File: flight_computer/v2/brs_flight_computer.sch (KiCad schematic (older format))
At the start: 0 parts

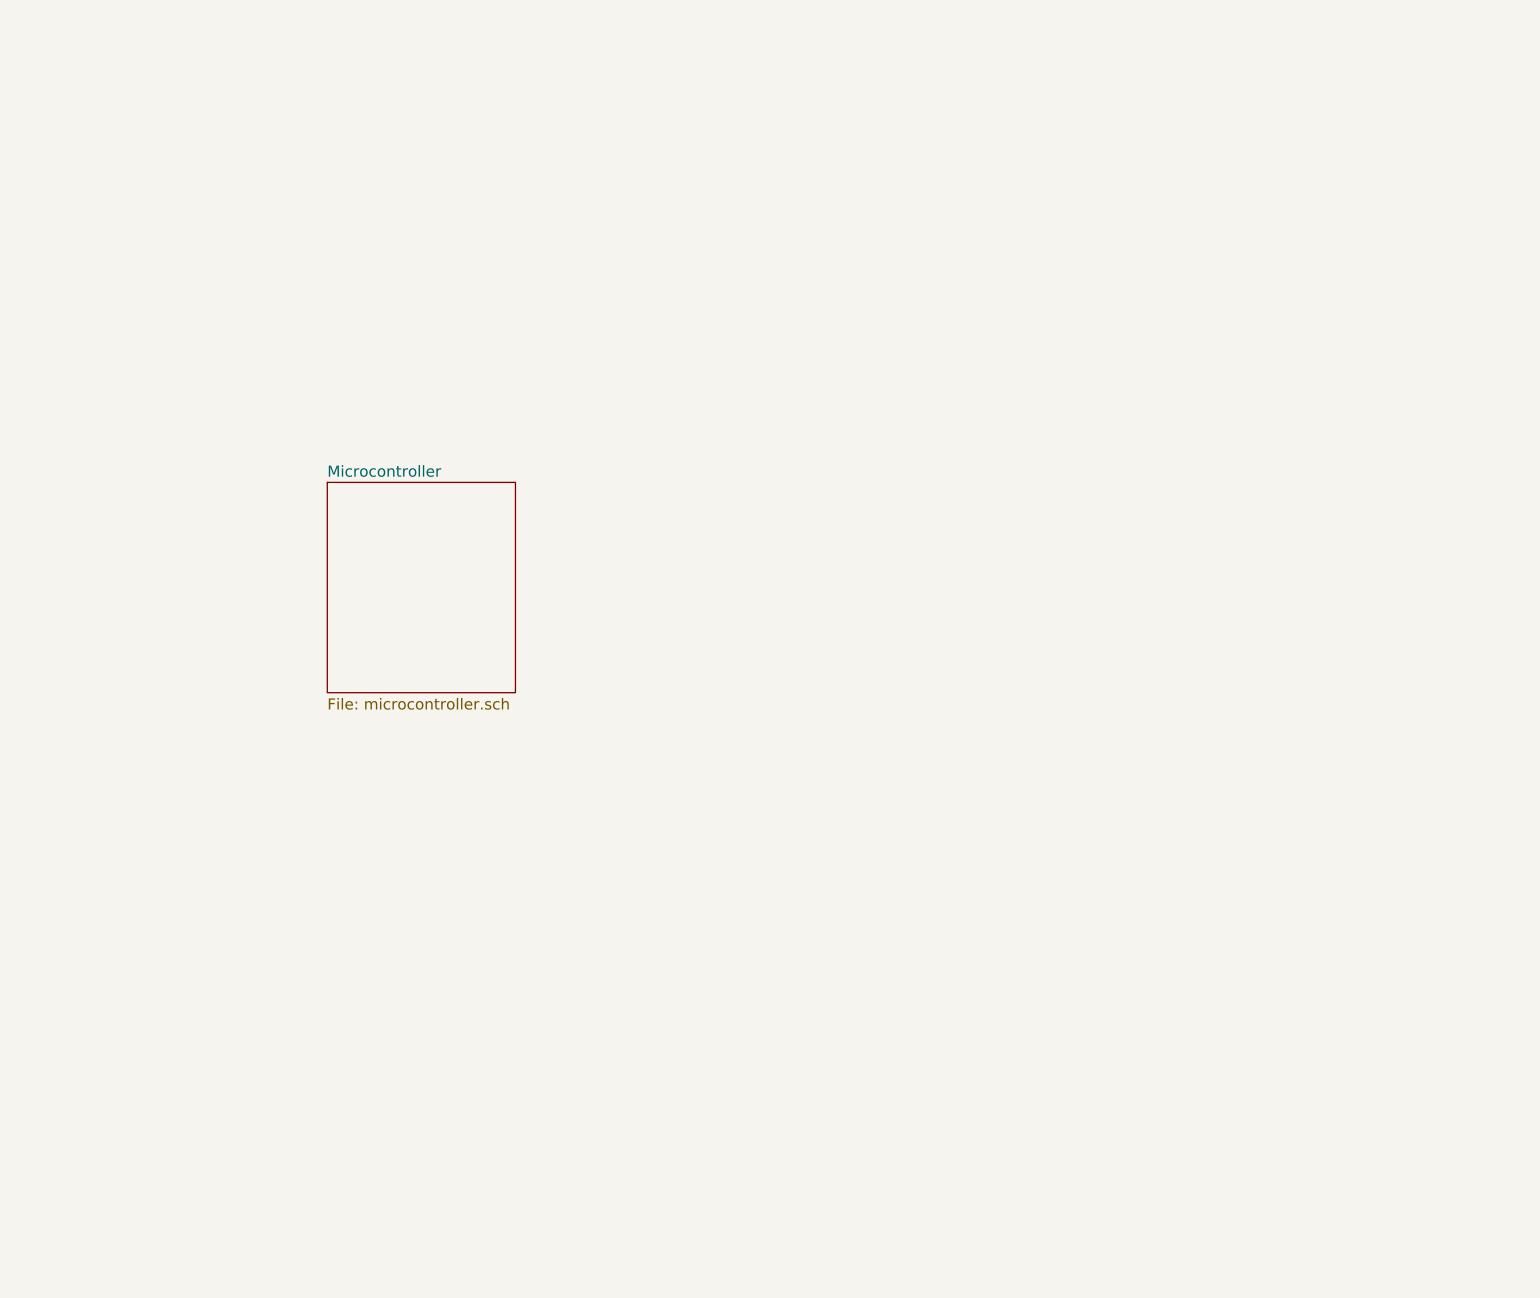
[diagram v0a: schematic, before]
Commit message: Nearing first pass layout for Rev B flight computer
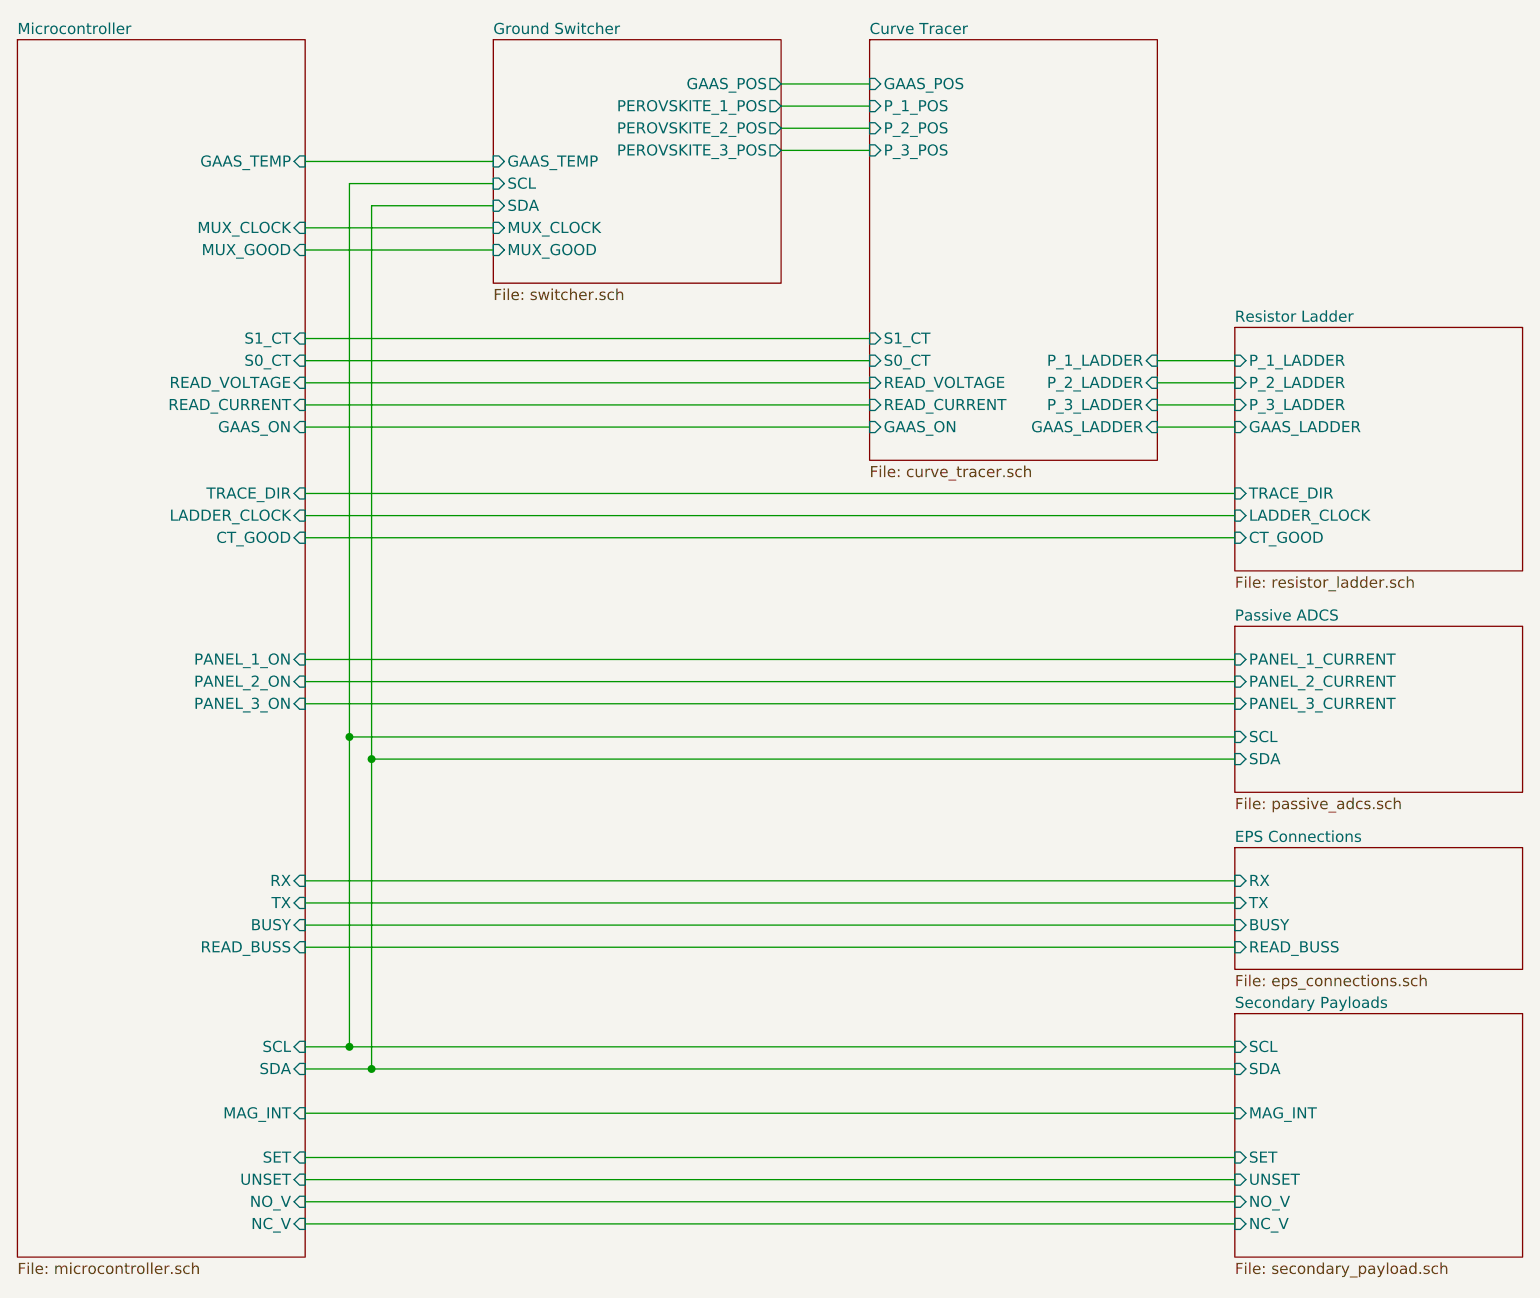
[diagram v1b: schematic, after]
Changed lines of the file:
@@
 $Descr A4 11693 8268
 encoding utf-8
-Sheet 1 2
-Title ""
-Date ""
-Rev ""
-Comp ""
-Comment1 ""
-Comment2 ""
-Comment3 ""
-Comment4 ""
+Sheet 1 8
+Title "Big Red Satellite Flight Computer - Top Level"
+Date "2023-08-13"
+Rev "B"
+Comp "UNL Aerospace Club | Advanced eXperimental Payloads"
+Comment1 "Copyright (c) 2023"
+Comment2 "Designer: WSA"
+Comment3 "Reviewer:"
+Comment4 "Approved:"
 $EndDescr
 $Sheet
-S 3850 2800 850  950
+S 2450 800  1300 5500
 U 64AE160A
 F0 "Microcontroller" 50
 F1 "microcontroller.sch" 50
-$EndSheet
+F2 "READ_CURRENT" I R 3750 2450 50
+F3 "READ_VOLTAGE" I R 3750 2350 50
+F4 "S0_CT" I R 3750 2250 50
+F5 "S1_CT" I R 3750 2150 50
+F6 "GAAS_ON" I R 3750 2550 50
+F7 "MUX_CLOCK" I R 3750 1650 50
+F8 "MUX_GOOD" I R 3750 1750 50
+F9 "GAAS_TEMP" I R 3750 1350 50
+F10 "LADDER_CLOCK" I R 3750 2950 50
+F11 "TRACE_DIR" I R 3750 2850 50
+F12 "CT_GOOD" I R 3750 3050 50
+F13 "PANEL_1_ON" I R 3750 3600 50
+F14 "PANEL_2_ON" I R 3750 3700 50
+F15 "PANEL_3_ON" I R 3750 3800 50
+F16 "SCL" I R 3750 5350 50
+F17 "SDA" I R 3750 5450 50
+F18 "BUSY" I R 3750 4800 50
+F19 "RX" I R 3750 4600 50
+F20 "TX" I R 3750 4700 50
+F21 "MAG_INT" I R 3750 5650 50
+F22 "SET" I R 3750 5850 50
+F23 "UNSET" I R 3750 5950 50
+F24 "NO_V" I R 3750 6050 50
+F25 "NC_V" I R 3750 6150 50
+F26 "READ_BUSS" I R 3750 4900 50
+$EndSheet
+$Sheet
+S 6300 800  1300 1900
+U 64D8220D
+F0 "Curve Tracer" 50
+F1 "curve_tracer.sch" 50
+F2 "GAAS_POS" I L 6300 1000 50
+F3 "GAAS_LADDER" I R 7600 2550 50
+F4 "GAAS_ON" I L 6300 2550 50
+F5 "P_1_POS" I L 6300 1100 50
+F6 "P_1_LADDER" I R 7600 2250 50
+F7 "P_2_POS" I L 6300 1200 50
+F8 "P_2_LADDER" I R 7600 2350 50
+F9 "P_3_POS" I L 6300 1300 50
+F10 "P_3_LADDER" I R 7600 2450 50
+F11 "READ_CURRENT" I L 6300 2450 50
+F12 "READ_VOLTAGE" I L 6300 2350 50
+F13 "S0_CT" I L 6300 2250 50
+F14 "S1_CT" I L 6300 2150 50
+$EndSheet
+$Sheet
+S 7950 3450 1300 750
+U 64D823E8
+F0 "Passive ADCS" 50
+F1 "passive_adcs.sch" 50
+F2 "PANEL_1_CURRENT" I L 7950 3600 50
+F3 "PANEL_2_CURRENT" I L 7950 3700 50
+F4 "PANEL_3_CURRENT" I L 7950 3800 50
+F5 "SCL" I L 7950 3950 50
+F6 "SDA" I L 7950 4050 50
+$EndSheet
+$Sheet
+S 7950 2100 1300 1100
+U 64D82674
+F0 "Resistor Ladder" 50
+F1 "resistor_ladder.sch" 50
+F2 "P_2_LADDER" I L 7950 2350 50
+F3 "P_3_LADDER" I L 7950 2450 50
+F4 "P_1_LADDER" I L 7950 2250 50
+F5 "GAAS_LADDER" I L 7950 2550 50
+F6 "LADDER_CLOCK" I L 7950 2950 50
+F7 "TRACE_DIR" I L 7950 2850 50
+F8 "CT_GOOD" I L 7950 3050 50
+$EndSheet
+$Sheet
+S 4600 800  1300 1100
+U 64D827F9
+F0 "Ground Switcher" 50
+F1 "switcher.sch" 50
+F2 "MUX_CLOCK" I L 4600 1650 50
+F3 "MUX_GOOD" I L 4600 1750 50
+F4 "PEROVSKITE_1_POS" O R 5900 1100 50
+F5 "PEROVSKITE_2_POS" O R 5900 1200 50
+F6 "PEROVSKITE_3_POS" O R 5900 1300 50
+F7 "GAAS_POS" O R 5900 1000 50
+F8 "SDA" I L 4600 1550 50
+F9 "SCL" I L 4600 1450 50
+F10 "GAAS_TEMP" I L 4600 1350 50
+$EndSheet
+Wire Wire Line
+	7950 2250 7600 2250
+Wire Wire Line
+	7600 2350 7950 2350
+Wire Wire Line
+	7950 2450 7600 2450
+Wire Wire Line
+	7600 2550 7950 2550
+Wire Wire Line
+	5900 1000 6300 1000
+Wire Wire Line
+	6300 1100 5900 1100
+Wire Wire Line
+	5900 1200 6300 1200
+Wire Wire Line
+	6300 1300 5900 1300
+$Sheet
+S 7950 4450 1300 550
+U 64D821F3
+F0 "EPS Connections" 50
+F1 "eps_connections.sch" 50
+F2 "RX" I L 7950 4600 50
+F3 "TX" I L 7950 4700 50
+F4 "BUSY" I L 7950 4800 50
+F5 "READ_BUSS" I L 7950 4900 50
+$EndSheet
+$Sheet
+S 7950 5200 1300 1100
+U 6685FD81
+F0 "Secondary Payloads" 50
+F1 "secondary_payload.sch" 50
+F2 "SCL" I L 7950 5350 50
+F3 "SDA" I L 7950 5450 50
+F4 "MAG_INT" I L 7950 5650 50
+F5 "SET" I L 7950 5850 50
+F6 "UNSET" I L 7950 5950 50
+F7 "NO_V" I L 7950 6050 50
+F8 "NC_V" I L 7950 6150 50
+$EndSheet
+Wire Wire Line
+	4600 1350 3750 1350
+Wire Wire Line
+	3750 1650 4600 1650
+Wire Wire Line
+	4600 1750 3750 1750
+Wire Wire Line
+	3750 2150 6300 2150
+Wire Wire Line
+	6300 2250 3750 2250
+Wire Wire Line
+	3750 2350 6300 2350
+Wire Wire Line
+	6300 2450 3750 2450
+Wire Wire Line
+	3750 2550 6300 2550
+Wire Wire Line
+	3750 2850 7950 2850
+Wire Wire Line
+	3750 2950 7950 2950
+Wire Wire Line
+	7950 3050 3750 3050
+Wire Wire Line
+	3750 3600 7950 3600
+Wire Wire Line
+	7950 3700 3750 3700
+Wire Wire Line
+	3750 3800 7950 3800
+Wire Wire Line
+	3750 4600 7950 4600
+Wire Wire Line
+	3750 4700 7950 4700
+Wire Wire Line
+	7950 4800 3750 4800
+Wire Wire Line
+	3750 5350 3950 5350
+Wire Wire Line
+	7950 5450 4050 5450
+Wire Wire Line
+	3750 5650 7950 5650
+Wire Wire Line
+	4600 1450 3950 1450
+Connection ~ 3950 5350
+Wire Wire Line
+	3950 5350 7950 5350
+Wire Wire Line
+	4600 1550 4050 1550
+Wire Wire Line
+	4050 1550 4050 4050
+Connection ~ 4050 5450
+Wire Wire Line
+	4050 5450 3750 5450
+Wire Wire Line
+	7950 3950 3950 3950
+Wire Wire Line
+	3950 1450 3950 3950
+Connection ~ 3950 3950
+Wire Wire Line
+	3950 3950 3950 5350
+Wire Wire Line
+	7950 4050 4050 4050
+Connection ~ 4050 4050
+Wire Wire Line
+	4050 4050 4050 5450
+Wire Wire Line
+	7950 5850 3750 5850
+Wire Wire Line
+	3750 5950 7950 5950
+Wire Wire Line
+	7950 6050 3750 6050
+Wire Wire Line
+	3750 6150 7950 6150
+Wire Wire Line
+	3750 4900 7950 4900
 $EndSCHEMATC

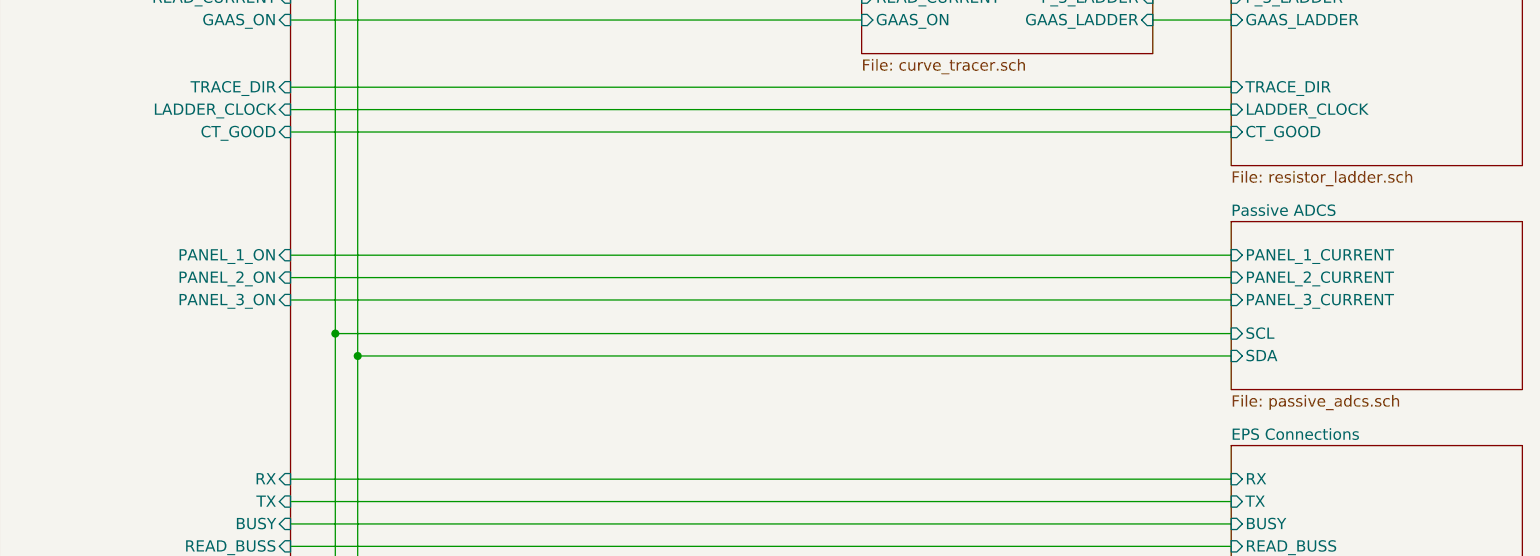
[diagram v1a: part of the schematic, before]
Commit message: Finished layout of flight computer
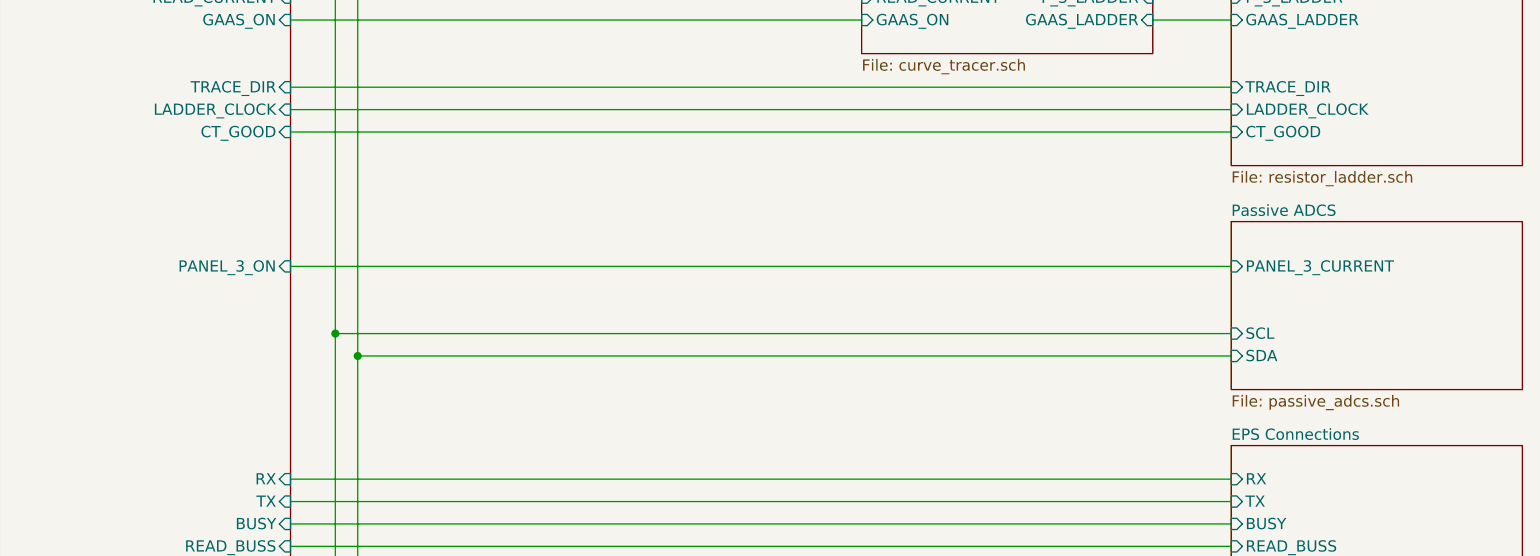
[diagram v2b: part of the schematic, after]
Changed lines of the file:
@@
 $EndDescr
-$Sheet
-S 2450 800  1300 5500
-U 64AE160A
-F0 "Microcontroller" 50
-F1 "microcontroller.sch" 50
-F2 "READ_CURRENT" I R 3750 2450 50
-F3 "READ_VOLTAGE" I R 3750 2350 50
-F4 "S0_CT" I R 3750 2250 50
-F5 "S1_CT" I R 3750 2150 50
-F6 "GAAS_ON" I R 3750 2550 50
-F7 "MUX_CLOCK" I R 3750 1650 50
-F8 "MUX_GOOD" I R 3750 1750 50
-F9 "GAAS_TEMP" I R 3750 1350 50
-F10 "LADDER_CLOCK" I R 3750 2950 50
-F11 "TRACE_DIR" I R 3750 2850 50
-F12 "CT_GOOD" I R 3750 3050 50
-F13 "PANEL_1_ON" I R 3750 3600 50
-F14 "PANEL_2_ON" I R 3750 3700 50
-F15 "PANEL_3_ON" I R 3750 3800 50
-F16 "SCL" I R 3750 5350 50
-F17 "SDA" I R 3750 5450 50
-F18 "BUSY" I R 3750 4800 50
-F19 "RX" I R 3750 4600 50
-F20 "TX" I R 3750 4700 50
-F21 "MAG_INT" I R 3750 5650 50
-F22 "SET" I R 3750 5850 50
-F23 "UNSET" I R 3750 5950 50
-F24 "NO_V" I R 3750 6050 50
-F25 "NC_V" I R 3750 6150 50
-F26 "READ_BUSS" I R 3750 4900 50
-$EndSheet
 $Sheet
 S 6300 800  1300 1900
@@
 F0 "Passive ADCS" 50
 F1 "passive_adcs.sch" 50
-F2 "PANEL_1_CURRENT" I L 7950 3600 50
-F3 "PANEL_2_CURRENT" I L 7950 3700 50
-F4 "PANEL_3_CURRENT" I L 7950 3800 50
-F5 "SCL" I L 7950 3950 50
-F6 "SDA" I L 7950 4050 50
+F2 "PANEL_3_CURRENT" I L 7950 3650 50
+F3 "SCL" I L 7950 3950 50
+F4 "SDA" I L 7950 4050 50
 $EndSheet
 $Sheet
@@
 	7950 3050 3750 3050
 Wire Wire Line
-	3750 3600 7950 3600
-Wire Wire Line
-	7950 3700 3750 3700
-Wire Wire Line
-	3750 3800 7950 3800
+	3750 3650 7950 3650
 Wire Wire Line
 	3750 4600 7950 4600
@@
 Wire Wire Line
 	3750 4900 7950 4900
+$Sheet
+S 2450 800  1300 5500
+U 64AE160A
+F0 "Microcontroller" 50
+F1 "microcontroller.sch" 50
+F2 "READ_CURRENT" I R 3750 2450 50
+F3 "READ_VOLTAGE" I R 3750 2350 50
+F4 "S0_CT" I R 3750 2250 50
+F5 "S1_CT" I R 3750 2150 50
+F6 "GAAS_ON" I R 3750 2550 50
+F7 "MUX_CLOCK" I R 3750 1650 50
+F8 "MUX_GOOD" I R 3750 1750 50
+F9 "GAAS_TEMP" I R 3750 1350 50
+F10 "LADDER_CLOCK" I R 3750 2950 50
+F11 "TRACE_DIR" I R 3750 2850 50
+F12 "CT_GOOD" I R 3750 3050 50
+F13 "PANEL_3_ON" I R 3750 3650 50
+F14 "SCL" I R 3750 5350 50
+F15 "SDA" I R 3750 5450 50
+F16 "BUSY" I R 3750 4800 50
+F17 "RX" I R 3750 4600 50
+F18 "TX" I R 3750 4700 50
+F19 "MAG_INT" I R 3750 5650 50
+F20 "SET" I R 3750 5850 50
+F21 "UNSET" I R 3750 5950 50
+F22 "NO_V" I R 3750 6050 50
+F23 "NC_V" I R 3750 6150 50
+F24 "READ_BUSS" I R 3750 4900 50
+$EndSheet
 $EndSCHEMATC
